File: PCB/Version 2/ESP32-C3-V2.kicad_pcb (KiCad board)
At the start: 4 copper layers, 28.1 x 24.4 mm, 50 parts, among them J2 DPS_PPS, J3 HCZZ0001-4, Q1 WPM2031-3/TR, SW2 TS-1187A-B-A-B, U1 USB-C-16P-SMD, U2 DS8561-33S5, U3 ESP32-C3, U4 BQ24073RGTR, U5 SKCL3130ME, Y1 40MHz_S3240000151040

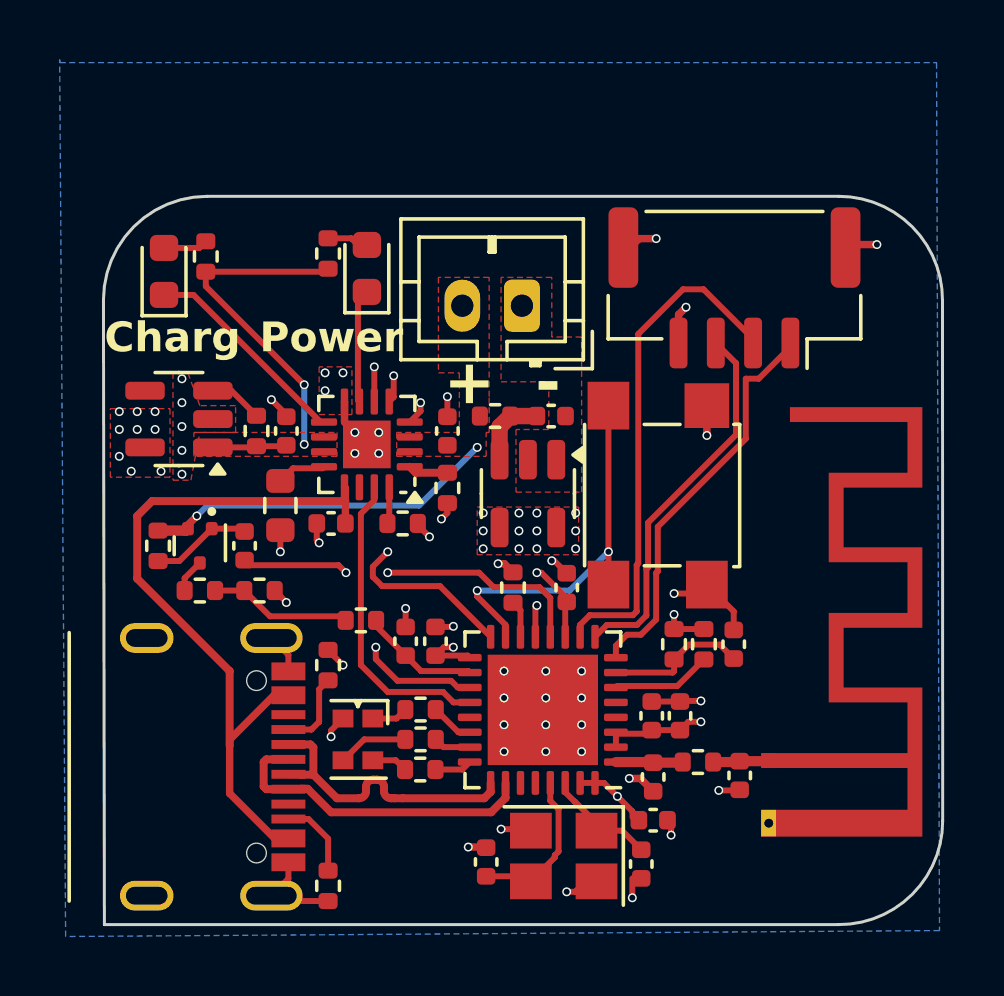
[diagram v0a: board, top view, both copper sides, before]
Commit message: neue Bilder, Gerber, PDF
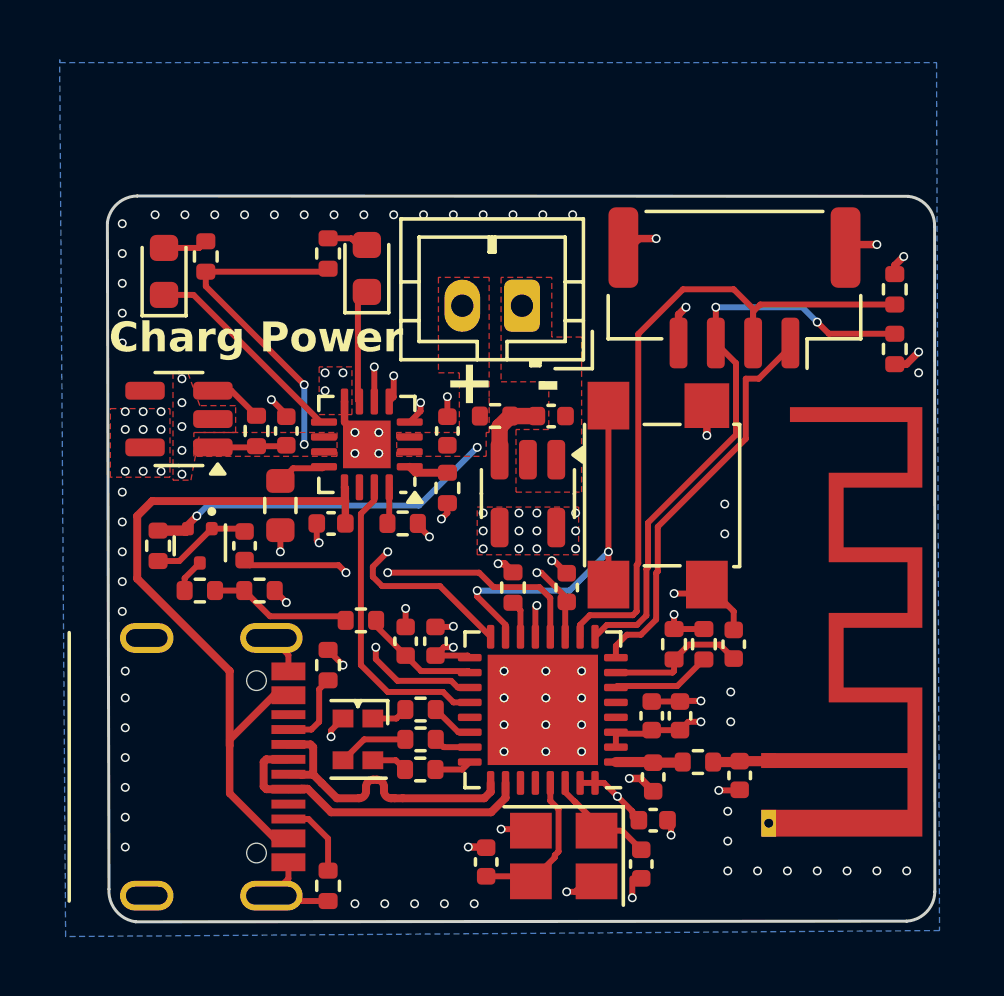
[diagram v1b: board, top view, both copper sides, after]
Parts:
- added R10: 5k1_0402, Resistor_SMD:R_0402_1005Metric, F.Cu at (155.5, 77.0)
- added R9: 5k1_0402, Resistor_SMD:R_0402_1005Metric, F.Cu at (155.5, 75.0)
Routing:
- net MCU_SCL: track 12.7 -> 20.2 mm, vias 0 -> 2
- net MCU_SDA: track 17.1 -> 23.6 mm
- net +3.3V: track 13.5 -> 15.2 mm, vias 16 -> 18
- net GND: vias 60 -> 111
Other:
- board size 28.1 x 24.4 mm -> 27.7 x 24.3 mm
